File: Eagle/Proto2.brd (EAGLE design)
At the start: 100 x 80 mm, 297 parts, among them Q1 310mA/60V/1.6Ω, Q10 310mA/60V/1.6Ω, Q129 310mA/60V/1.6Ω, Q13 310mA/60V/1.6Ω, Q130 310mA/60V/1.6Ω, Q131 310mA/60V/1.6Ω, Q132 310mA/60V/1.6Ω, Q133 310mA/60V/1.6Ω, Q134 310mA/60V/1.6Ω, Q135 310mA/60V/1.6Ω, Q136 310mA/60V/1.6Ω, Q137 310mA/60V/1.6Ω, Q138 310mA/60V/1.6Ω, Q139 310mA/60V/1.6Ω, Q14 310mA/60V/1.6Ω, Q140 310mA/60V/1.6Ω, Q141 310mA/60V/1.6Ω, Q142 310mA/60V/1.6Ω, Q143 310mA/60V/1.6Ω, Q144 310mA/60V/1.6Ω, Q145 310mA/60V/1.6Ω, Q146 310mA/60V/1.6Ω, Q147 310mA/60V/1.6Ω, Q148 310mA/60V/1.6Ω, Q149 310mA/60V/1.6Ω, Q150 310mA/60V/1.6Ω, Q151 310mA/60V/1.6Ω, Q152 310mA/60V/1.6Ω, Q153 310mA/60V/1.6Ω, Q154 310mA/60V/1.6Ω, Q155 310mA/60V/1.6Ω, Q156 310mA/60V/1.6Ω, Q157 310mA/60V/1.6Ω, Q158 310mA/60V/1.6Ω, Q159 310mA/60V/1.6Ω, Q160 310mA/60V/1.6Ω, Q17 310mA/60V/1.6Ω, Q18 310mA/60V/1.6Ω, Q193 310mA/60V/1.6Ω, Q194 310mA/60V/1.6Ω, Q195 310mA/60V/1.6Ω, Q196 310mA/60V/1.6Ω, Q197 310mA/60V/1.6Ω, Q198 310mA/60V/1.6Ω, Q199 310mA/60V/1.6Ω, Q2 310mA/60V/1.6Ω, Q200 310mA/60V/1.6Ω, Q201 310mA/60V/1.6Ω, Q202 310mA/60V/1.6Ω, Q203 310mA/60V/1.6Ω, Q204 310mA/60V/1.6Ω, Q205 310mA/60V/1.6Ω, Q206 310mA/60V/1.6Ω, Q207 310mA/60V/1.6Ω, Q208 310mA/60V/1.6Ω, Q209 310mA/60V/1.6Ω, Q21 310mA/60V/1.6Ω, Q210 310mA/60V/1.6Ω, Q211 310mA/60V/1.6Ω, Q212 310mA/60V/1.6Ω, Q213 310mA/60V/1.6Ω, Q214 310mA/60V/1.6Ω, Q215 310mA/60V/1.6Ω, Q216 310mA/60V/1.6Ω, Q217 310mA/60V/1.6Ω, Q218 310mA/60V/1.6Ω, Q219 310mA/60V/1.6Ω, Q22 310mA/60V/1.6Ω, Q220 310mA/60V/1.6Ω, Q221 310mA/60V/1.6Ω, Q222 310mA/60V/1.6Ω, Q223 310mA/60V/1.6Ω, Q224 310mA/60V/1.6Ω, Q25 310mA/60V/1.6Ω, Q257 310mA/60V/1.6Ω, Q258 310mA/60V/1.6Ω, Q259 310mA/60V/1.6Ω, Q26 310mA/60V/1.6Ω, Q260 310mA/60V/1.6Ω, Q261 310mA/60V/1.6Ω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

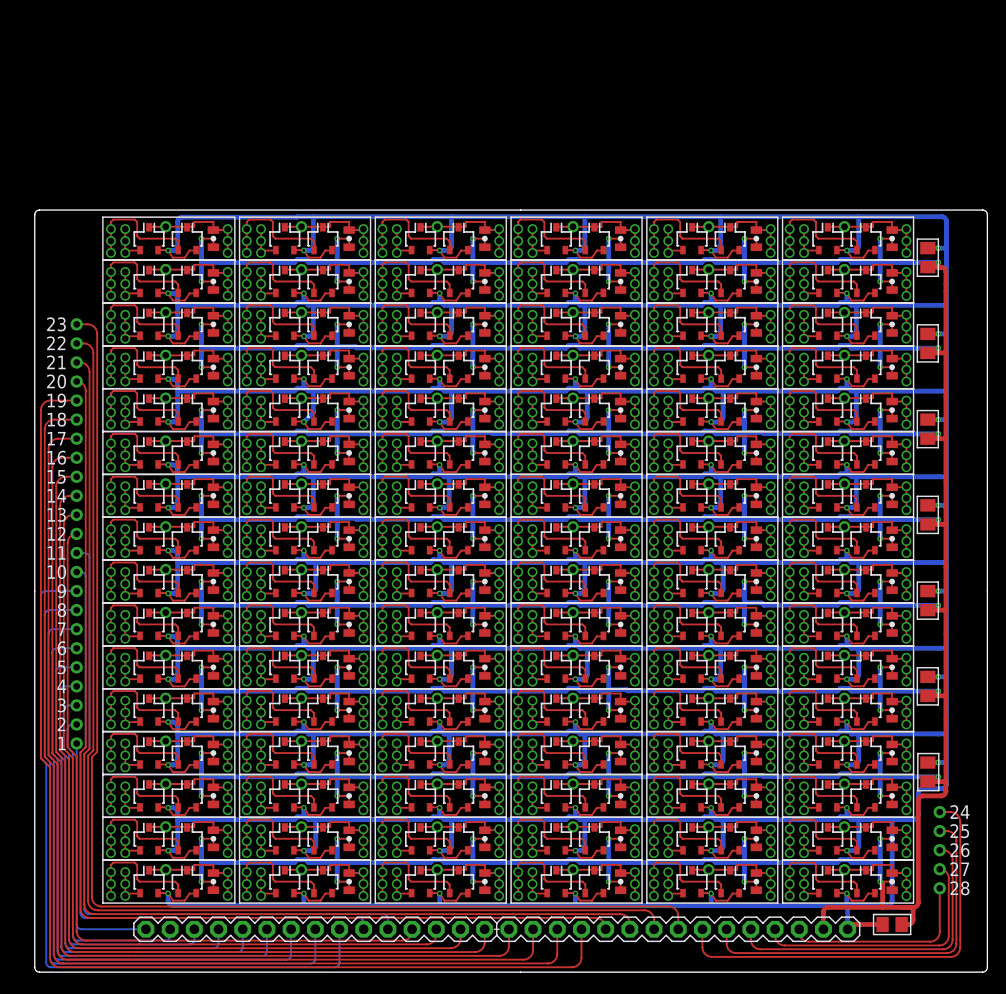
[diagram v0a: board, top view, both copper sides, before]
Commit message: Updated boards with pcb template
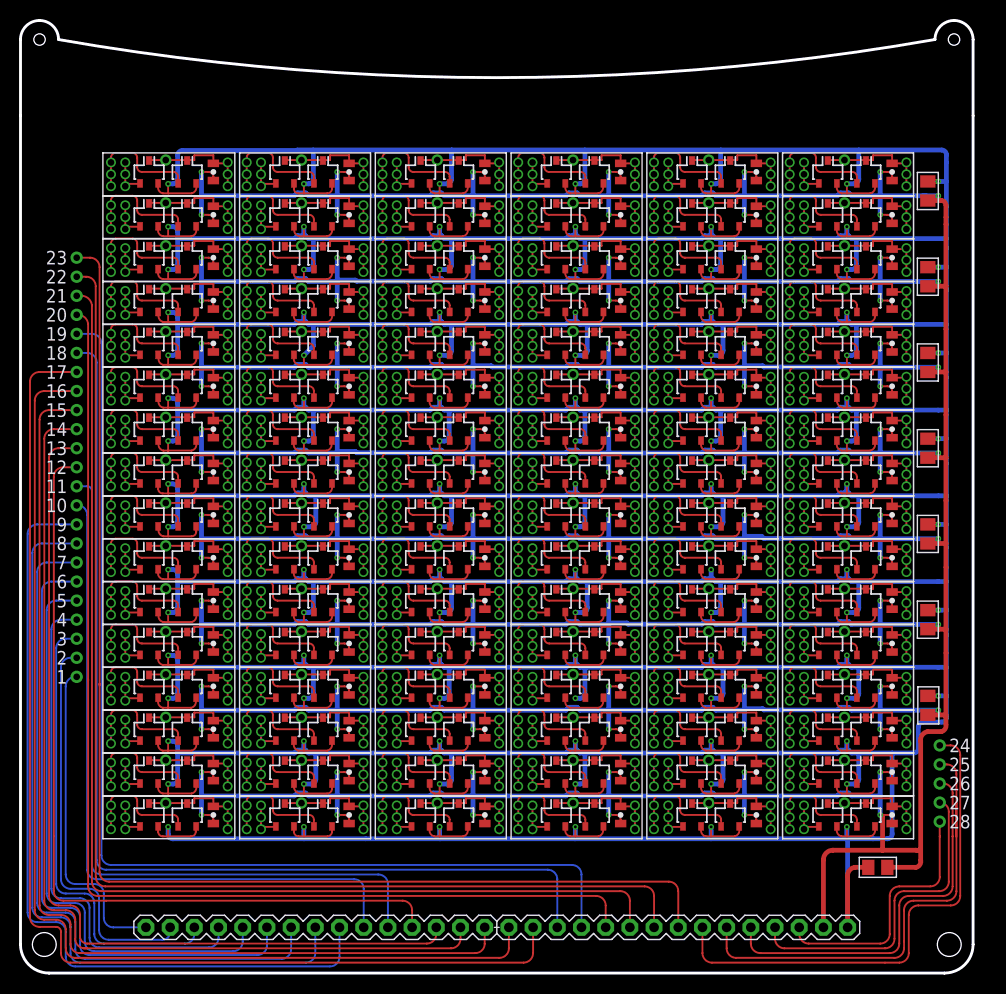
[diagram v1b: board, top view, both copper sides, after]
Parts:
- moved C10 7.00 mm to (93.8, 55.0)
- moved C12 7.00 mm to (93.8, 64.0)
- moved C14 7.00 mm to (93.8, 73.0)
- moved C16 7.00 mm to (93.8, 82.0)
- moved C4 7.00 mm to (93.8, 28.0)
- moved C6 7.00 mm to (93.8, 37.0)
- moved C8 7.00 mm to (93.8, 46.0)
- moved Q1 7.00 mm to (12.0, 16.5)
- moved Q10 7.00 mm to (16.0, 25.5)
- moved Q129 7.00 mm to (40.5, 16.5)
- moved Q13 7.00 mm to (12.0, 30.0)
- moved Q130 7.00 mm to (44.5, 16.5)
- moved Q131 7.00 mm to (40.5, 21.0)
- moved Q132 7.00 mm to (44.5, 21.0)
- moved Q133 7.00 mm to (40.5, 25.5)
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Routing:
- net GND: track 1536.7 -> 1695.6 mm
- net N$2: track 1261.0 -> 1207.5 mm
- net VCC: track 1150.1 -> 1131.3 mm
- net P17: track 109.4 -> 120.8 mm
- net P16: track 103.2 -> 114.1 mm
- net P25: track 39.4 -> 50.0 mm
- net P15: track 97.1 -> 107.4 mm
- net P14: track 91.0 -> 101.3 mm
- net P13: track 84.8 -> 94.5 mm
- net P9: track 77.4 -> 85.6 mm
- net P19: track 121.7 -> 113.5 mm
- net P8: track 71.2 -> 79.1 mm
- net P12: track 78.7 -> 86.6 mm
- net P7: track 65.1 -> 72.8 mm
- net P6: track 59.0 -> 66.4 mm
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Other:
- board size 100 x 80 mm -> 100 x 100 mm
- board text added: "NOR2 proto rev1"
- board text removed: "Dual NOR proto Rev 1"
